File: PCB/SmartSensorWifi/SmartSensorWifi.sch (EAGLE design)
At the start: 7 parts, among them IC1 AT45DB-S

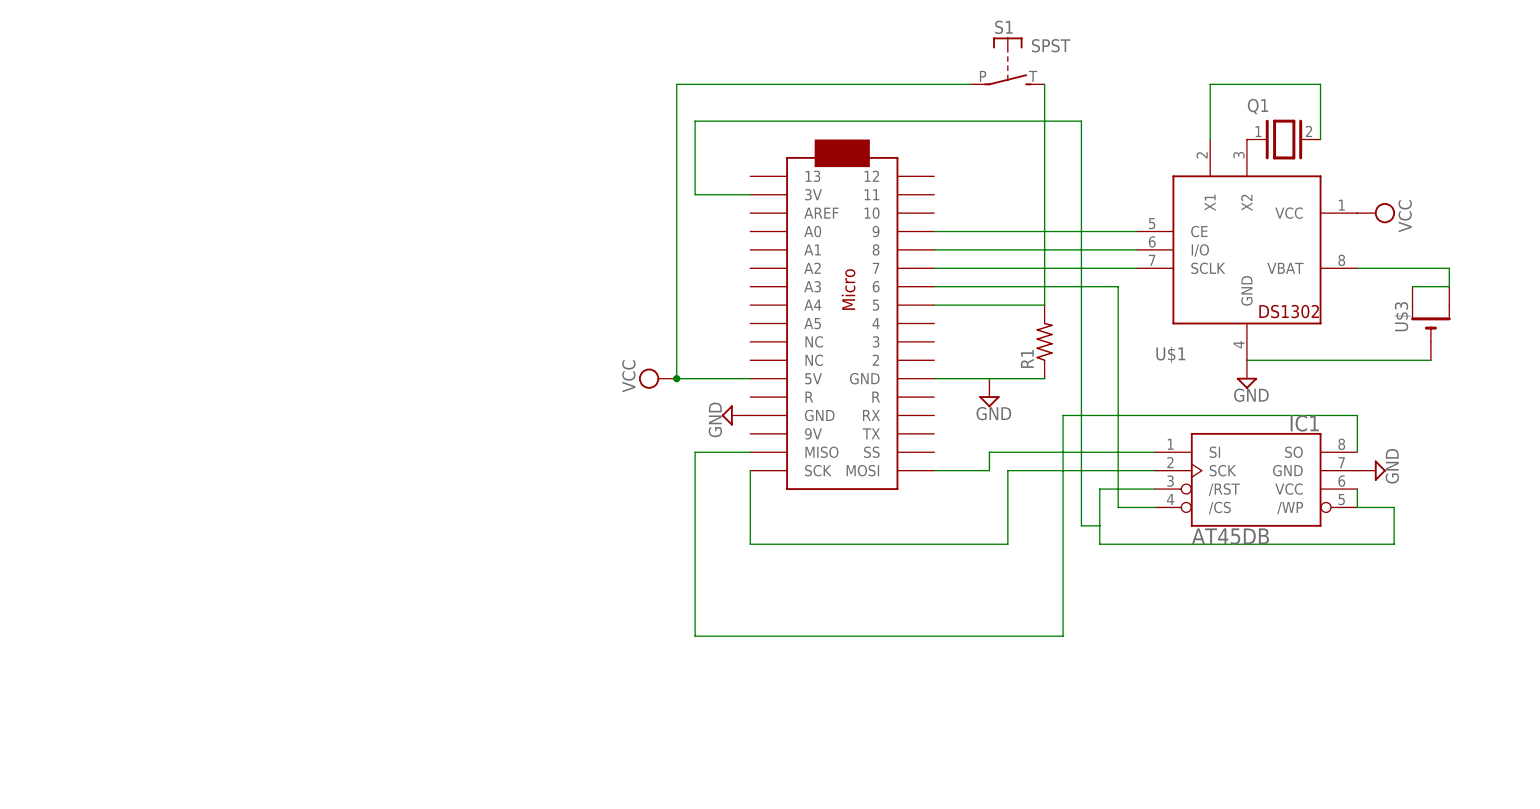
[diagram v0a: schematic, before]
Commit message: Updated the eagle files
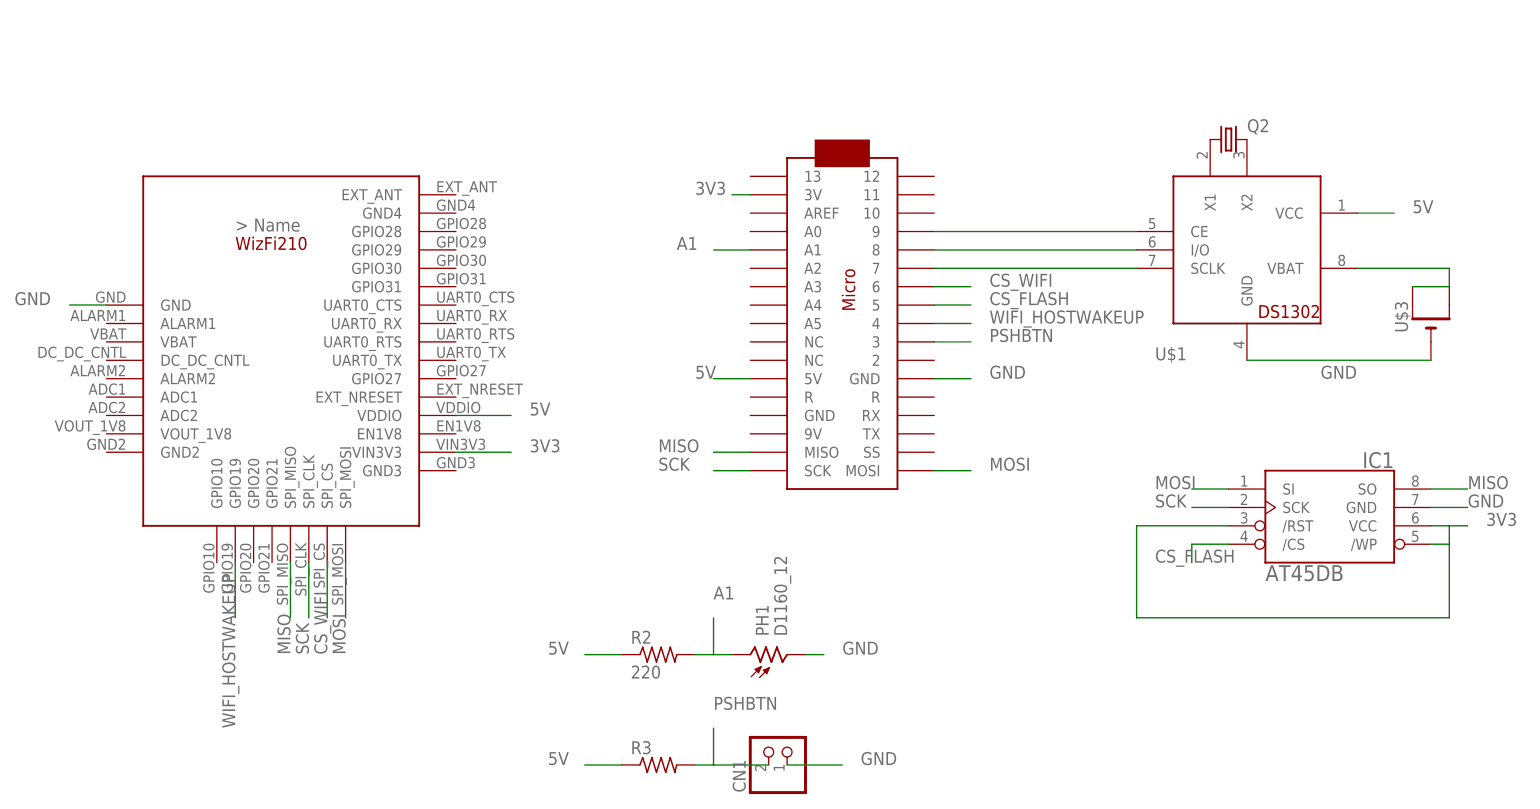
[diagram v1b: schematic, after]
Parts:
- removed Q1: (no value), special:XTAL
- removed R1: (no value), adafruit:R-US_0204/7
- removed S1: SPST, adafruit:SPST
- added CN1: (no value), adafruit:JST_2PIN-THM
- added PH1: D1160_12, photo-elements:D1160_12
- added Q2: (no value), adafruit:CRYSTALTC38H
- added R2: 220, adafruit:R-US_0207/12
- added R3: (no value), adafruit:R-US_0207/12
- added U$4: WIZFISTACKED, SmartSensorWifi:WIZFISTACKED
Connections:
- removed net N$11: IC1./CS, U$2.6
- removed net N$12: R1.2, S1.S, U$2.5
- removed net N$6: IC1.SO, U$2.MISO
- removed net N$7: IC1.SCK, U$2.SCK
- removed net N$8: IC1.SI, U$2.MOSI
- removed net N$9: IC1./RST, IC1./WP, IC1.VCC, U$2.3V
- removed net VCC: S1.P, U$1.VCC, U$2.5V
- new net 3V3: IC1./RST, IC1./WP, IC1.VCC, U$2.3V, U$4.VIN3V3
- new net 5V: R2.1, R3.1, U$1.VCC, U$2.5V, U$4.VDDIO
- new net A1: PH1.1, R2.2, U$2.A1
- new net CS_FLASH: IC1./CS, U$2.5
- new net CS_WIFI: U$2.6, U$4.SPI_CS
- new net MISO: IC1.SO, U$2.MISO, U$4.SPI_MISO
- new net MOSI: IC1.SI, U$2.MOSI, U$4.SPI_MOSI
- new net PSHBTN: CN1.1, R3.2, U$2.3
- new net SCK: IC1.SCK, U$2.SCK, U$4.SPI_CLK
- new net WIFI_HOSTWAKEUP: U$2.4, U$4.GPIO19
- net GND: now also CN1.2, PH1.2, U$4.GND; no longer R1.1, U$2.GND
- net N$2: now also Q2.2; no longer Q1.1
- net N$3: now also Q2.1; no longer Q1.2
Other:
- moved on the sheet: IC1
